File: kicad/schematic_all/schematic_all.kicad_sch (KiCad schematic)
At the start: 43 parts, among them SW1 Bourns PEC11R, SW2 SW_Push, SW3 Bourns PEC11R, U1 RPi_Pico_TH, U2 RDA5807M_Module, U3 LM386, U4 LM386

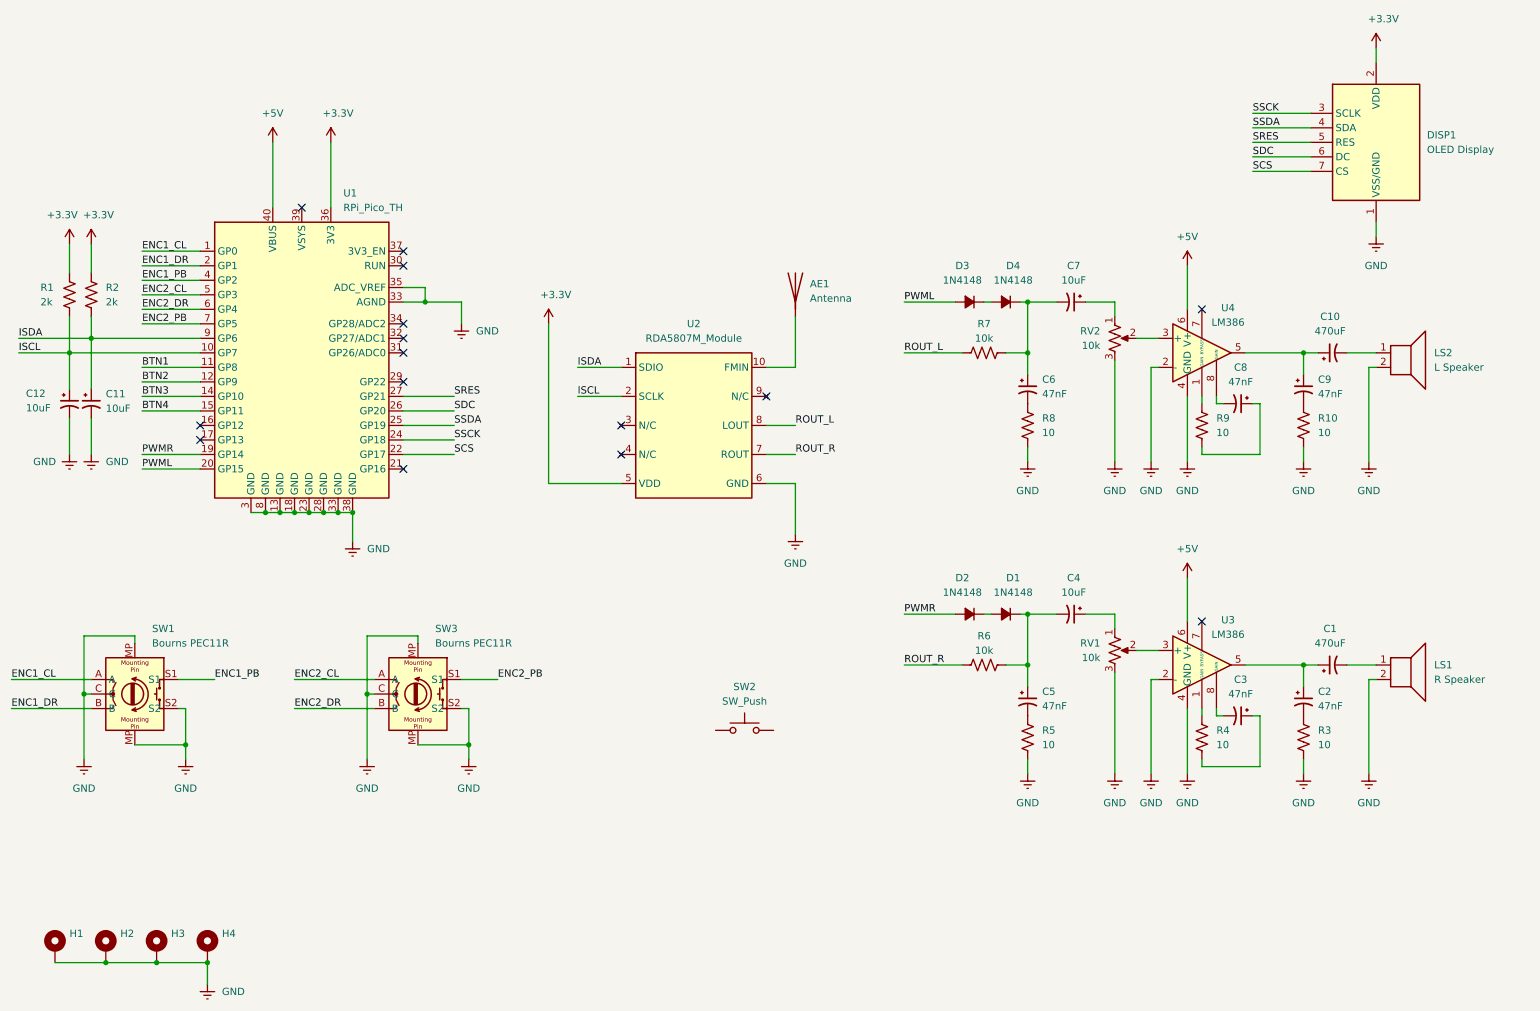
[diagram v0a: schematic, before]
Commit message: schematic v0.1
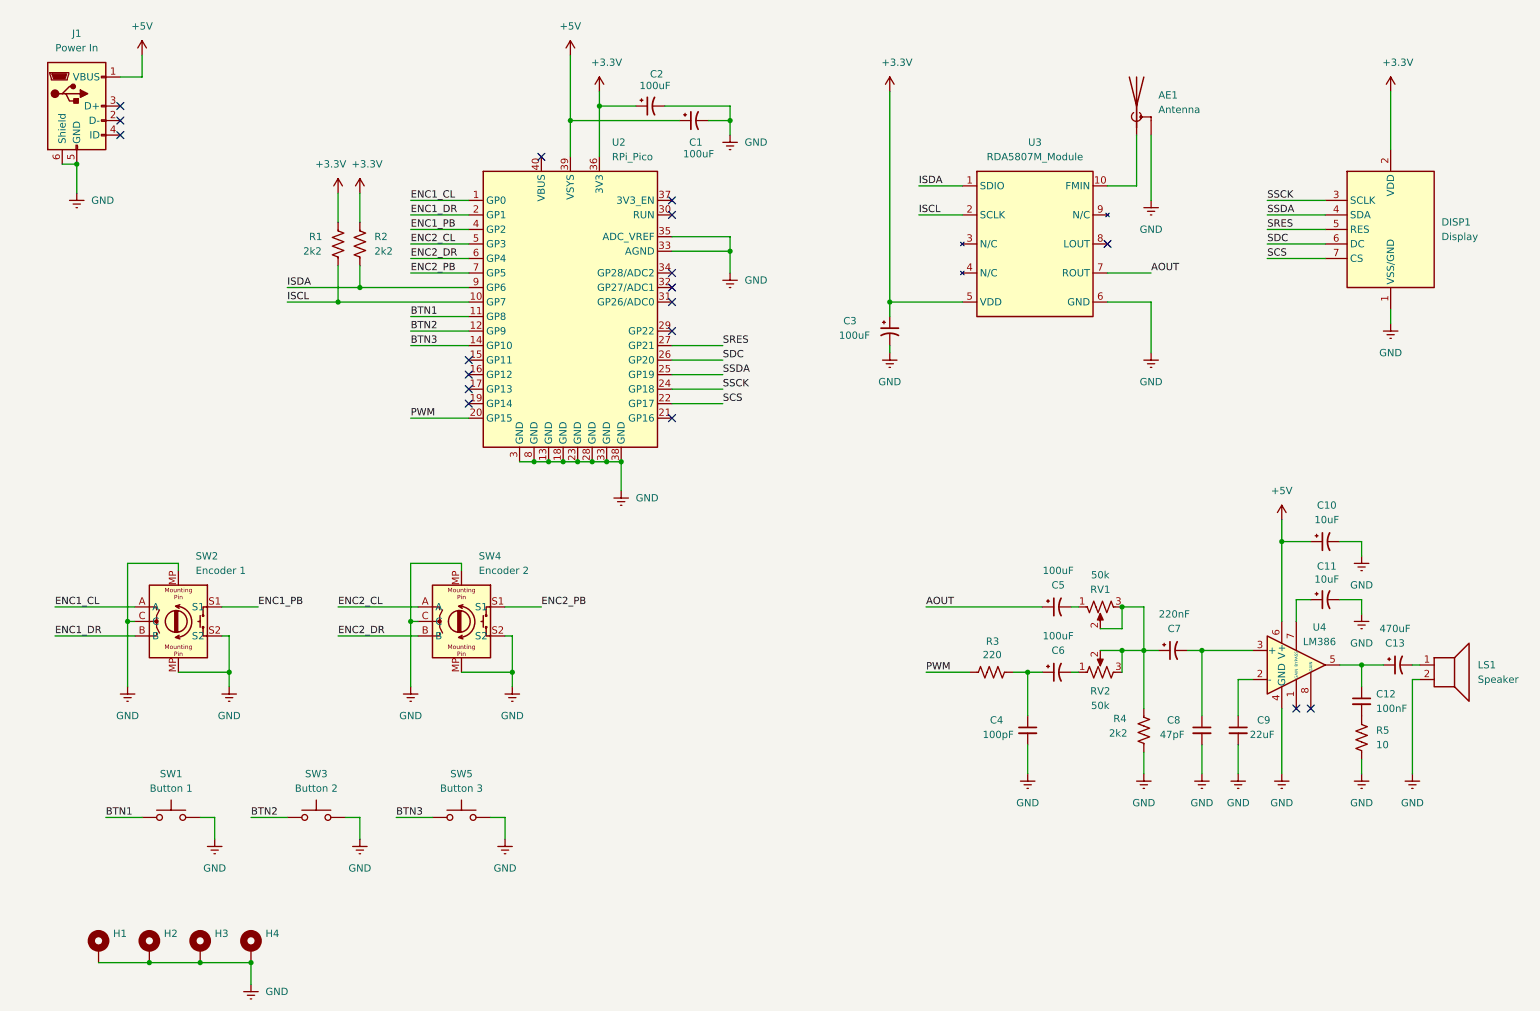
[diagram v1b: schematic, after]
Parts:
- removed AE1: Antenna, symbol Device:Antenna
- removed C12, C7: 10uF, symbol Device:C_Polarized_Small_US
- removed C8, C9: 47nF, symbol Device:C_Polarized_Small_US
- removed D1, D2, D3, D4: 1N4148, symbol Device:D_Small_Filled
- removed LS2: L Speaker, symbol Device:Speaker
- removed R10, R5, R8, R9: 10, symbol Device:R_US
- removed R6, R7: 10k, symbol Device:R_US
- removed U4: LM386, symbol Amplifier_Audio:LM386
- added AE1: Antenna, TerminalBlock_Phoenix:TerminalBlock_Phoenix_MKDS-1,5-2_1x02_P5.00mm_Horizontal, symbol Device:Antenna_Shield
- added C1, C2: 100uF, Capacitor_THT:CP_Radial_D5.0mm_P2.00mm, symbol Device:C_Polarized_Small_US
- added C4: 100pF, Capacitor_THT:CP_Radial_D5.0mm_P2.00mm, symbol Device:C_Small
- added C8: 47pF, Capacitor_THT:C_Rect_L7.0mm_W2.5mm_P5.00mm, symbol Device:C_Small
- added C9: 22uF, Capacitor_THT:CP_Radial_D5.0mm_P2.00mm, symbol Device:C_Small
- added J1: Power In, TerminalBlock_Phoenix:TerminalBlock_Phoenix_MKDS-1,5-2_1x02_P5.00mm_Horizontal, symbol Connector:USB_B_Micro
- added R3: 220, Resistor_THT:R_Axial_DIN0207_L6.3mm_D2.5mm_P10.16mm_Horizontal, symbol Device:R_US
- added SW3: Button 2, TerminalBlock_Phoenix:TerminalBlock_Phoenix_MKDS-1,5-2_1x02_P5.00mm_Horizontal, symbol Switch:SW_Push
- added SW5: Button 3, TerminalBlock_Phoenix:TerminalBlock_Phoenix_MKDS-1,5-2_1x02_P5.00mm_Horizontal, symbol Switch:SW_Push
- C10: value 470uF -> 10uF; footprint (none) -> Capacitor_THT:CP_Radial_D5.0mm_P2.00mm
- C11: footprint (none) -> Capacitor_THT:CP_Radial_D5.0mm_P2.00mm
- C12: renamed from C2; value 47nF -> 100nF; footprint (none) -> Capacitor_THT:CP_Radial_D5.0mm_P2.00mm; symbol Device:C_Polarized_Small_US -> Device:C_Small
- C13: renamed from C1; footprint (none) -> Capacitor_THT:CP_Radial_D6.3mm_P2.50mm
- C3, C5, C6: value 47nF -> 100uF; footprint (none) -> Capacitor_THT:CP_Radial_D5.0mm_P2.00mm
- C7: renamed from C4; value 10uF -> 220nF; footprint (none) -> Capacitor_THT:CP_Radial_D5.0mm_P2.00mm
- DISP1: value OLED Display -> Display; footprint (none) -> TerminalBlock_Phoenix:TerminalBlock_Phoenix_MKDS-1,5-7_1x07_P5.00mm_Horizontal
- H1, H2, H3, H4: footprint (none) -> MountingHole:MountingHole_3.2mm_M3_Pad
- LS1: value R Speaker -> Speaker; footprint (none) -> TerminalBlock_Phoenix:TerminalBlock_Phoenix_MKDS-1,5-2_1x02_P5.00mm_Horizontal
- R1, R2: value 2k -> 2k2; footprint (none) -> Resistor_THT:R_Axial_DIN0207_L6.3mm_D2.5mm_P10.16mm_Horizontal
- R4: value 10 -> 2k2; footprint (none) -> Resistor_THT:R_Axial_DIN0207_L6.3mm_D2.5mm_P10.16mm_Horizontal
- R5: renamed from R3; footprint (none) -> Resistor_THT:R_Axial_DIN0207_L6.3mm_D2.5mm_P10.16mm_Horizontal
- RV1, RV2: value 10k -> 50k; footprint (none) -> ECE:Bourns_PTV09_Horiz
- SW1: renamed from SW2; value SW_Push -> Button 1; footprint (none) -> TerminalBlock_Phoenix:TerminalBlock_Phoenix_MKDS-1,5-2_1x02_P5.00mm_Horizontal
- SW2: renamed from SW1; value Bourns PEC11R -> Encoder 1; footprint Rotary_Encoder:RotaryEncoder_Alps_EC12E-Switch_Vertical_H20mm -> TerminalBlock_Phoenix:TerminalBlock_Phoenix_MKDS-1,5-4_1x04_P5.00mm_Horizontal
- SW4: renamed from SW3; value Bourns PEC11R -> Encoder 2; footprint Rotary_Encoder:RotaryEncoder_Alps_EC12E-Switch_Vertical_H20mm -> TerminalBlock_Phoenix:TerminalBlock_Phoenix_MKDS-1,5-4_1x04_P5.00mm_Horizontal
- U2: renamed from U1; value RPi_Pico_TH -> RPi_Pico
- U4: renamed from U3; footprint (none) -> Package_DIP:DIP-8_W7.62mm_Socket
- renumbered U2 to U3
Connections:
- net +3.3V: now also C3.1, C2.1
- net +5V: now also C10.1, U2.39 (VSYS), C1.1, J1.1 (VBUS); no longer U2.40 (VBUS)
- net BTN1: now also SW1.1
- net BTN2: now also SW3.1
- net BTN3: now also SW5.1
- net GND: now also C10.2, C3.2, R4.2, SW1.2, AE1.2 (Shield), C1.2, C2.2, C4.2, C8.2, C9.2, J1.5 (GND), J1.6 (Shield), SW3.2, SW5.2; no longer RV1.3, RV2.3, U4.2 (-)
- net ISDA: no longer C11.1
- net at R4.1: now also C7.1, RV1.2, RV1.3, RV2.2, RV2.3; no longer U4.1 (GAIN)
- net at U3.10 (FMIN): now also AE1.1 (A)
- net at C7.2: now also U4.3 (+), C8.1; no longer C5.1
- net at C6.1: now also C4.1, R3.1
- net at RV1.1: now also C5.2; no longer C7.1
- net at RV2.1: now also C6.2
- net at U4.7 (BYPASS): now also C11.1
- net at U4.8 (GAIN): no longer C3.2
- net BTN4: no longer names the net of U2.15 (GP11)
- net PWML renamed PWM
- net PWM: now also R3.2
- net PWMR: no longer names the net of U2.19 (GP14)
- net ROUT_L: no longer names the net of U3.8 (LOUT)
- net ROUT_R renamed AOUT
- net AOUT: now also C5.1
- new net: C9.1, U4.2 (-)
- no-connect marks 15 -> 18
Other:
- moved on the sheet: C13, C7, DISP1, H1, H2, H3, H4, LS1, R1, R2, R5, SW1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
